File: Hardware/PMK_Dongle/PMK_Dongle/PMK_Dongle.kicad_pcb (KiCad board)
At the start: 4 copper layers, 10.4 x 20.1 mm, 31 parts, among them IC1 ESP32-S2FH4, J1 USB_A, U1 MIC5528-3.3YMT-T5, Y1 40MHz

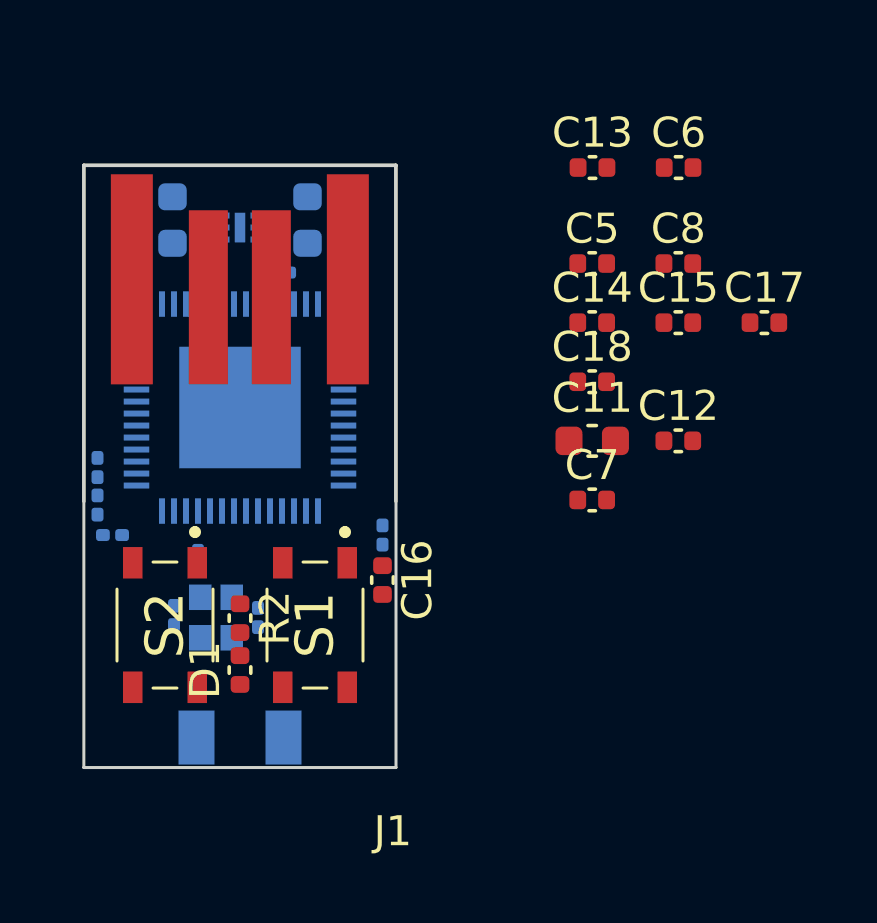
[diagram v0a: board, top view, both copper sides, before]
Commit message: Layout is almost done
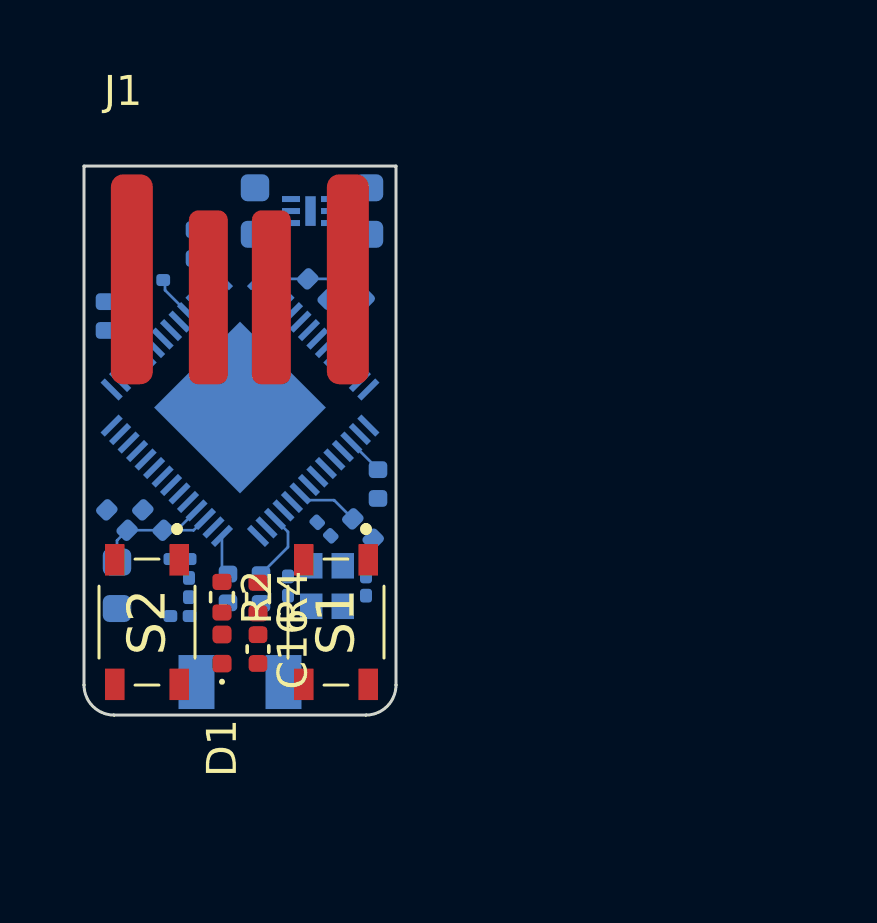
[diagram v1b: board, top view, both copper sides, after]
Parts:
- C11, C12, C13, C14, C15, C17, C18, C5, C6, C7, C8: moved to B.Cu
- D1: footprint Capacitor_SMD:C_0402_1005Metric -> LED_SMD:LED_0402_1005Metric
- L1: footprint Capacitor_SMD:C_0201_0603Metric -> Inductor_SMD:L_0201_0603Metric
- R1, R3: footprint Capacitor_SMD:C_0201_0603Metric -> Resistor_SMD:R_0201_0603Metric
- R2: footprint Capacitor_SMD:C_0402_1005Metric -> Resistor_SMD:R_0402_1005Metric
- R4: footprint Capacitor_SMD:C_0201_0603Metric -> Resistor_SMD:R_0402_1005Metric; moved to F.Cu
- moved C17 22.0 mm to (148.5, 38.2), turned to 90 degrees
- moved C6 19.8 mm to (153.7, 47.3), turned to -90 degrees
- moved C12 18.9 mm to (148.9, 45.0), turned to 135 degrees
- moved C13 18.8 mm to (150.1, 45.0), turned to 135 degrees
- moved C8 18.5 mm to (152.6, 47.3), turned to -90 degrees
- moved C11 16.6 mm to (148.9, 47.2), turned to -90 degrees
- moved C18 14.0 mm to (151.5, 35.8), turned to 90 degrees
- moved C15 10.9 mm to (156.8, 37.3), turned to -45 degrees
- moved C5 10.2 mm to (157.6, 43.8), turned to -90 degrees
- moved C14 9.21 mm to (155.6, 37.3), turned to -45 degrees
- moved C7 7.70 mm to (157.1, 45.3), turned to -45 degrees
- moved C16 4.74 mm to (153.6, 49.3)
- moved R4 4.65 mm to (153.6, 47.6)
- moved R1 4.33 mm to (155.8, 45.3), turned to 135 degrees
- moved R3 4.21 mm to (150.1, 37.0), turned to 0 degrees
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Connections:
- R2 pad 1: /IO15 -> /IO46
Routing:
- net +3V3: track 0.00 -> 15.6 mm
- net /VDD_SPI: track 0.00 -> 2.70 mm
- net /IO18: track 0.00 -> 1.40 mm
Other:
- board size 10.4 x 20.1 mm -> 10.4 x 18.3 mm

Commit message: Routing ongoing
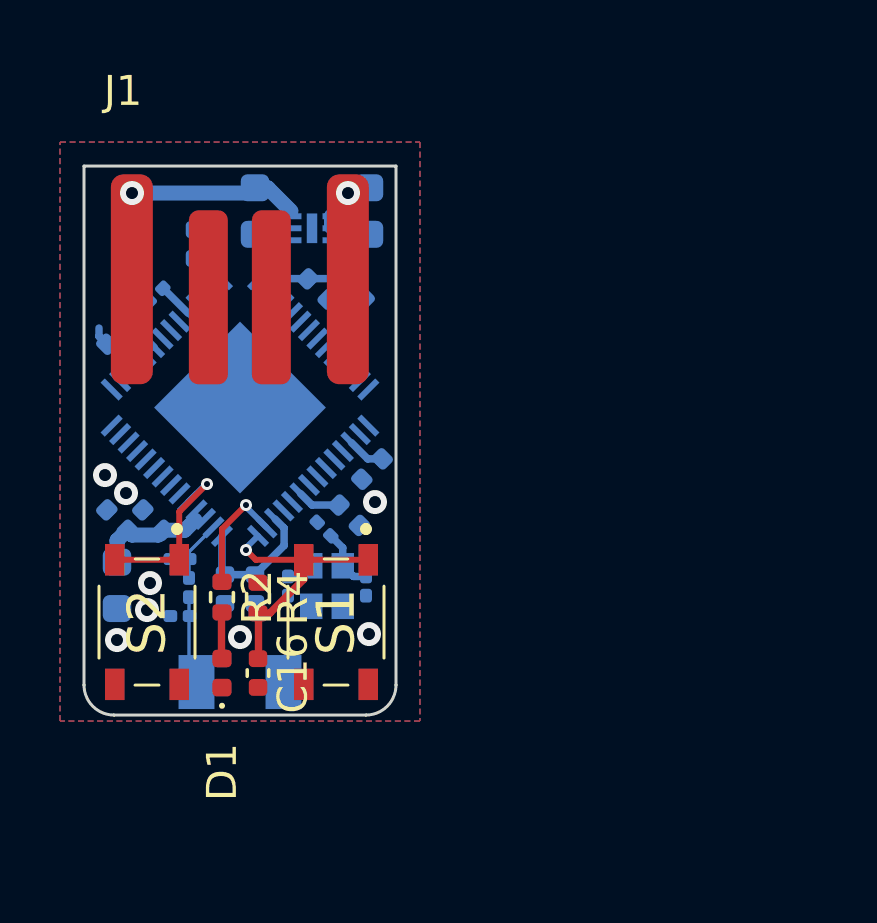
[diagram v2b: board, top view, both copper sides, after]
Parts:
- moved C16 0.80 mm to (153.6, 50.1)
- moved D1 0.80 mm to (152.4, 50.1)
- moved C17 0.72 mm to (148.9, 38.8), turned to -135 degrees
- moved C7 0.65 mm to (156.6, 44.8)
- moved U1 0.58 mm to (155.4, 35.3)
- moved C5 0.54 mm to (157.4, 43.3), turned to -135 degrees
- moved R3 0.51 mm to (150.2, 37.5), turned to 45 degrees
- moved C6 0.20 mm to (153.5, 47.3)
- moved C8 0.10 mm to (152.5, 47.3)
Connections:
- S1 pad 3: (no net) -> /EN
- S2 pad 3: (no net) -> /IO0
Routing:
- net /EN: track 0.00 -> 9.02 mm, vias 0 -> 1
- net VBUS: track 0.00 -> 7.20 mm, vias 0 -> 1
- net /IO0: track 0.00 -> 5.94 mm, vias 0 -> 1
- net /IO46: track 0.00 -> 3.92 mm, vias 0 -> 1
- net Net-(ANT1-Pad1): track 0.00 -> 2.93 mm
- net /QUARTZ_1: track 0.00 -> 2.09 mm
- net /LNA_IN: track 0.00 -> 2.02 mm
- net Net-(D1-Pad2): track 0.00 -> 1.55 mm
- net GND: track 0.00 -> 1.42 mm, vias 0 -> 9
- net +3V3: track 15.6 -> 16.5 mm
- net /QUARTZ_2: track 0.00 -> 0.92 mm
- added copper zone on B.Cu, net GND
- added copper zone on F.Cu, net GND
- added copper zone on In1.Cu, net GND
- added copper zone on In2.Cu, net GND
